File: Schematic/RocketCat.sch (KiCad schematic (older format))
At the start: 3 parts

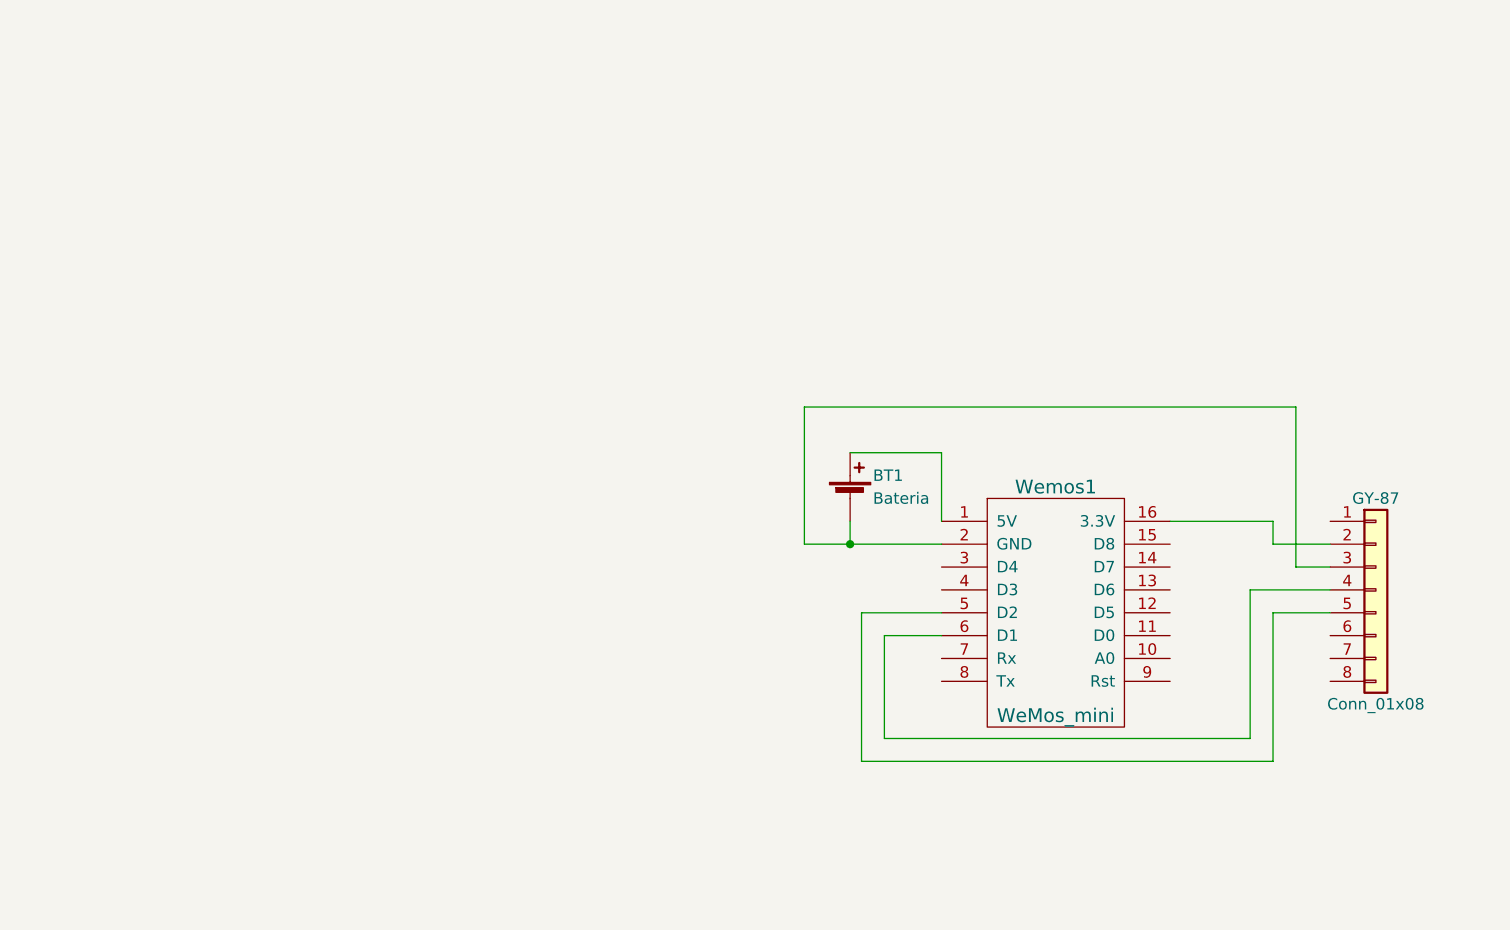
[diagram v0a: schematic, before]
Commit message: PCB Lista
Checar si no tengo nada mal
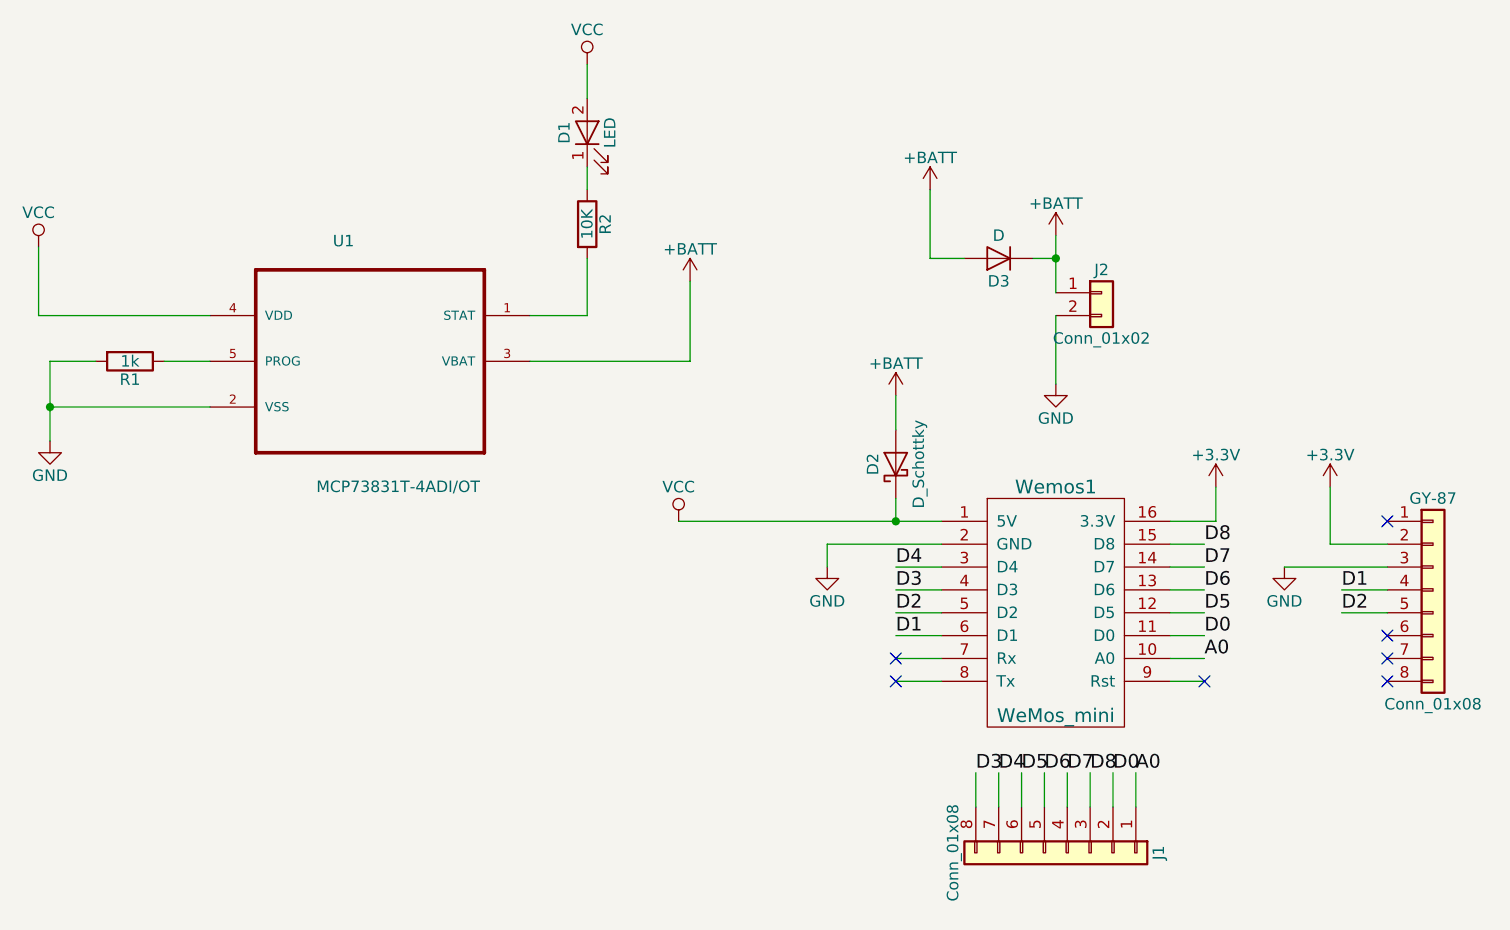
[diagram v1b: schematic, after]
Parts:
- removed BT1: Bateria, Battery_Holders:Keystone_1042_1x18650, symbol Battery_Cell
- added D1: LED, LEDs:LED_0805, symbol LED
- added D2: D_Schottky, Diodes_SMD:D_0805, symbol D_Schottky
- added D3: D, Diodes_SMD:D_0805, symbol D
- added J1: Conn_01x08, Socket_Strips:Socket_Strip_Straight_1x08_Pitch2.54mm, symbol Conn_01x08
- added J2: Conn_01x02, Socket_Strips:Socket_Strip_Straight_1x02_Pitch2.54mm, symbol Conn_01x02
- added R1: 1k, Resistors_SMD:R_0805, symbol R
- added R2: 10K, Resistors_SMD:R_0805, symbol R
- added U1: MCP73831T-4ADI/OT, TO_SOT_Packages_SMD:SOT-23-5, symbol MCP73831T-4ADI/OT
- GY-87: footprint Connectors:Wafer_Horizontal22.5x5.8x7RM2.5-8 -> Socket_Strips:Socket_Strip_Straight_1x08_Pitch2.54mm
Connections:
- net VCC: now reaches Wemos1.1 (5V)
- net VCC: now also D1.2 (A), D2.1 (K), U1.4 (VDD)
- net A0: now reaches Wemos1.10 (A0)
- net A0: now also J1.1 (Pin_1)
- net D0: now reaches Wemos1.11 (D0)
- net D0: now also J1.2 (Pin_2)
- net D5: now reaches Wemos1.12 (D5)
- net D5: now also J1.6 (Pin_6)
- net D6: now reaches Wemos1.13 (D6)
- net D6: now also J1.5 (Pin_5)
- net D7: now reaches Wemos1.14 (D7)
- net D7: now also J1.4 (Pin_4)
- net D8: now reaches Wemos1.15 (D8)
- net D8: now also J1.3 (Pin_3)
- net +3V3: now reaches GY-87.2 (Pin_2), Wemos1.16 (3.3V)
- net GND: now reaches GY-87.3 (Pin_3), Wemos1.2 (GND)
- net GND: now also J2.2 (Pin_2), R1.2, U1.2 (VSS)
- net D4: now reaches Wemos1.3 (D4)
- net D4: now also J1.7 (Pin_7)
- net D3: now reaches Wemos1.4 (D3)
- net D3: now also J1.8 (Pin_8)
- net D2: now reaches GY-87.5 (Pin_5), Wemos1.5 (D2)
- net D1: now reaches GY-87.4 (Pin_4), Wemos1.6 (D1)
- new net: R2.2, U1.1 (STAT)
- new net: R1.1, U1.5 (PROG)
- new net: D1.1 (K), R2.1
- new net +BATT: D2.2 (A), D3.1 (K), D3.2 (A), J2.1 (Pin_1), U1.3 (VBAT)
- no-connect marks 0 -> 7
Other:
- moved on the sheet: GY-87
